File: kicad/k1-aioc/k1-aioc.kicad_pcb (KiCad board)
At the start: 2 copper layers, 21 x 31.5 mm, 47 parts, among them J1 12401832E402A, J2 Conn_01x07_Male, Q1 BC847BS, U1 MIC5330-SSYML, U2 STM32F373CBTx, Y1 8MHz/20pF

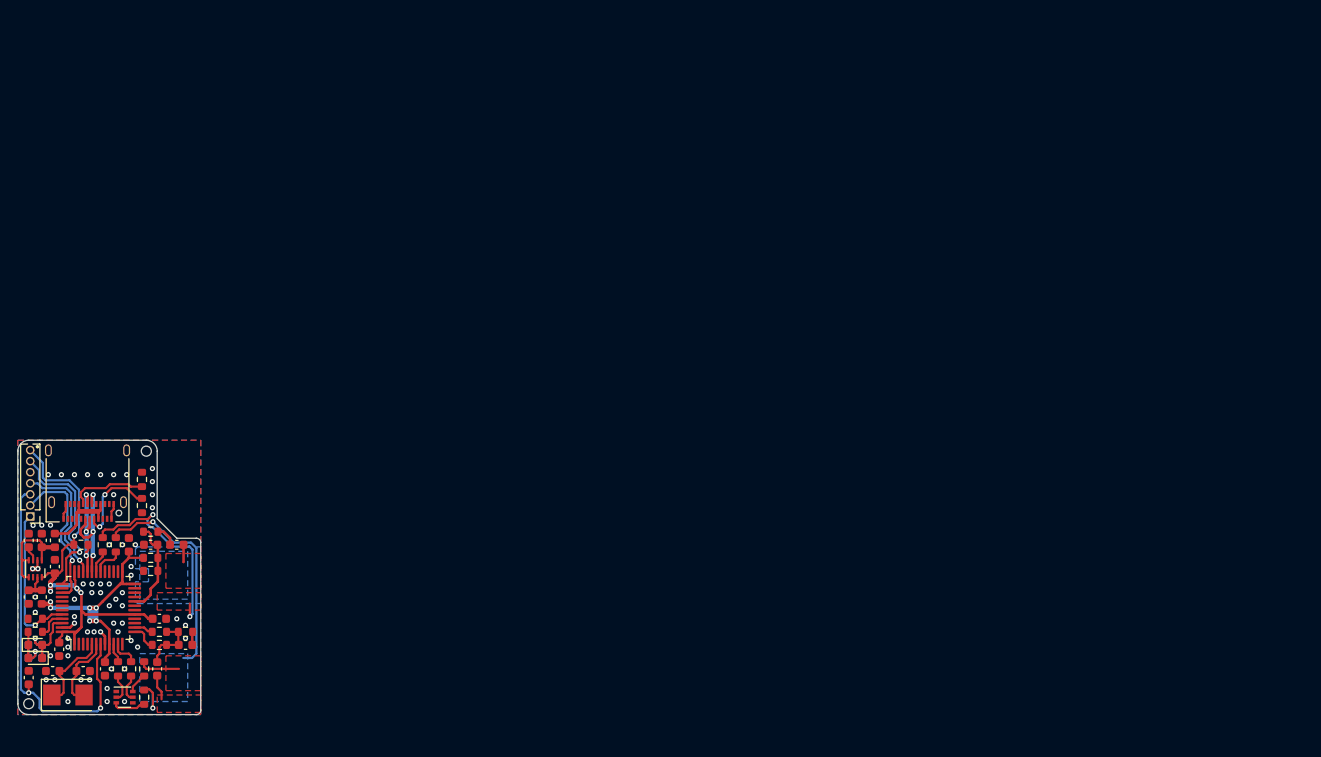
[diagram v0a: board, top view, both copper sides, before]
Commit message: Extensive PCB rework for new form factor
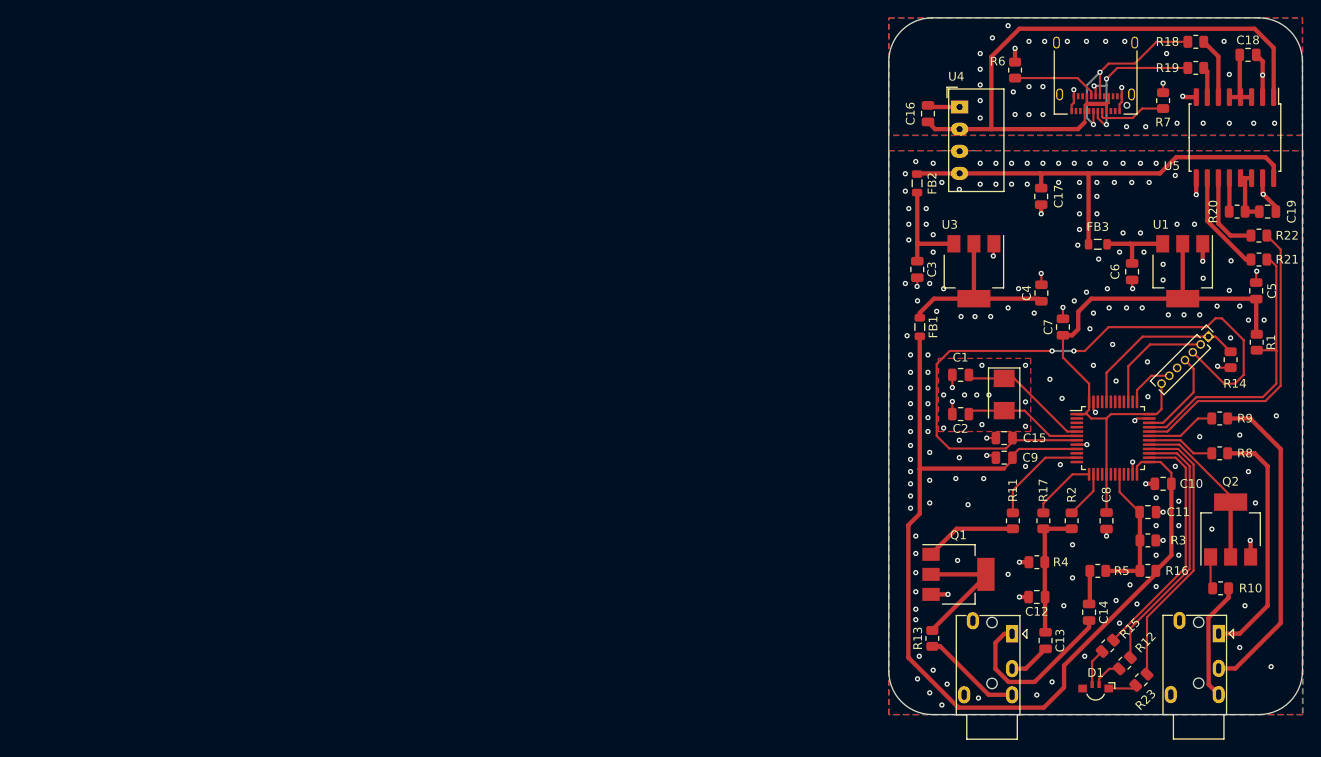
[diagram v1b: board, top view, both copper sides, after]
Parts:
- removed D2: RED, LED_SMD:LED_0603_1608Metric
- removed D3, D4: N.M., LED_SMD:LED_0603_1608Metric
- removed H1, H2: ToolingHole, AIOC:TOOLING-HOLE
- removed REF**: OSHW-Logo2_9.8x8mm_SilkScreen, Symbol:OSHW-Logo2_9.8x8mm_SilkScreen
- added C16: 4.7u/10V/X5R, Capacitor_SMD:C_0805_2012Metric, F.Cu at (208.0, 42.5)
- added C17: 4.7u/10V/X5R, Capacitor_SMD:C_0805_2012Metric, F.Cu at (221.0, 52.0)
- added C18: 100n, Capacitor_SMD:C_0805_2012Metric, F.Cu at (244.8, 35.8)
- added C19: 100n, Capacitor_SMD:C_0805_2012Metric, F.Cu at (247.0, 53.8)
- added FB2: 600R@100MHz, Inductor_SMD:L_0805_2012Metric, F.Cu at (206.8, 50.5)
- added J3: AUDIO, Connector_Audio:Jack_3.5mm_PJ320E_Horizontal, F.Cu at (217.7, 102.2)
- added J4: CAT, Connector_Audio:Jack_3.5mm_PJ320E_Horizontal, F.Cu at (241.4, 102.2)
- added Q2: PZT2222A, Package_TO_SOT_SMD:SOT-223-3_TabPin2, F.Cu at (242.8, 90.2)
- added R18: 24, Resistor_SMD:R_0805_2012Metric, F.Cu at (238.8, 34.2)
- added R19: 24, Resistor_SMD:R_0805_2012Metric, F.Cu at (238.8, 37.2)
- added R20: 5.1K, Resistor_SMD:R_0805_2012Metric, F.Cu at (243.5, 53.8)
- added R21: 24, Resistor_SMD:R_0805_2012Metric, F.Cu at (246.0, 59.2)
- added R22: 24, Resistor_SMD:R_0805_2012Metric, F.Cu at (246.0, 56.5)
- added R23: 220R, Resistor_SMD:R_0805_2012Metric, F.Cu at (232.5, 107.5)
- added U3: TLV1117LV-33, Package_TO_SOT_SMD:SOT-223-3_TabPin2, F.Cu at (213.3, 60.6)
- added U4: CRE1S0505SC, Converter_DCDC:Converter_DCDC_Murata_CRE1xxxxxxSC_THT, F.Cu at (211.6, 41.7)
- added U5: ADUM3160, Package_SO:SOIC-16W_7.5x10.3mm_P1.27mm, F.Cu at (243.2, 45.2)
- C1, C10, C11, C12, C13, C14, C15, C2, C4, C5, C6, C8, C9: footprint Capacitor_SMD:C_0603_1608Metric -> Capacitor_SMD:C_0805_2012Metric
- C3: value 100n -> 4.7u/10V/X5R; footprint Capacitor_SMD:C_0603_1608Metric -> Capacitor_SMD:C_0805_2012Metric
- C7: value 4.7u/10V/X5R -> 100n; footprint Capacitor_SMD:C_0603_1608Metric -> Capacitor_SMD:C_0805_2012Metric
- D1: value GREEN -> LED_RGBK; footprint LED_SMD:LED_0603_1608Metric -> LED_SMD:LED_Kingbright_APFA3010_3x1.5mm_Horizontal
- FB1: footprint Inductor_SMD:L_0603_1608Metric -> Inductor_SMD:L_0805_2012Metric
- FB3: renamed from FB2; footprint Inductor_SMD:L_0603_1608Metric -> Inductor_SMD:L_0805_2012Metric
- Q1: value BC847BS -> PZT2222A; footprint Package_TO_SOT_SMD:SOT-363_SC-70-6 -> Package_TO_SOT_SMD:SOT-223-3_TabPin2
- R1, R11, R14, R15, R16, R17, R2, R3, R4, R5, R6, R7, R8, R9: footprint Resistor_SMD:R_0603_1608Metric -> Resistor_SMD:R_0805_2012Metric
- R10: value 2.2K -> 24R; footprint Resistor_SMD:R_0603_1608Metric -> Resistor_SMD:R_0805_2012Metric
- R12: value 22R -> 220R; footprint Resistor_SMD:R_0603_1608Metric -> Resistor_SMD:R_0805_2012Metric
- R13: value 22R -> 24R; footprint Resistor_SMD:R_0603_1608Metric -> Resistor_SMD:R_0805_2012Metric
- U1: value MIC5330-SSYML -> TLV1117LV-33; footprint AIOC:Micrel_MLF-8-1EP_2x2mm_P0.5mm_EP0.6x1.2mm -> Package_TO_SOT_SMD:SOT-223-3_TabPin2
- moved C5 145.3 mm to (245.7, 62.8), turned to 90 degrees
- moved R14 140.4 mm to (242.8, 70.8), turned to 90 degrees
- moved R1 137.0 mm to (245.8, 68.8), turned to -90 degrees
- moved J2 136.8 mm to (240.2, 68.1), turned to -45 degrees
- moved U1 136.1 mm to (237.2, 60.6)
- moved R9 129.1 mm to (241.5, 77.5), turned to 180 degrees
- moved C6 128.9 mm to (231.4, 60.6), turned to -90 degrees
- moved R8 127.2 mm to (241.5, 81.5), turned to 180 degrees
- moved R10 126.9 mm to (241.6, 97.0), turned to 180 degrees
- moved R7 126.1 mm to (235.0, 41.0), turned to -90 degrees
- moved J1 124.9 mm to (227.2, 38.2)
- moved FB3 124.5 mm to (227.5, 57.5), turned to 180 degrees
- moved R15 123.2 mm to (228.6, 103.6), turned to 45 degrees
- moved D1 121.9 mm to (227.2, 108.5), turned to 180 degrees
- moved C8 121.2 mm to (228.5, 89.2)
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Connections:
- C4 pad 1: +3V3 -> Net-(C4-Pad1)
- C5 pad 1: Net-(C5-Pad1) -> +3V3
- C6 pad 1: /VIN -> Net-(C6-Pad1)
- D1 pad 2: Net-(D1-Pad2) -> GND
- FB1 pad 1: +3.3VA -> Net-(C4-Pad1)
- FB1 pad 2: Net-(C5-Pad1) -> +3.3VA
- FB3 pad 1: /VIN -> Net-(C6-Pad1)
- FB3 pad 2: /VBUS -> Net-(C17-Pad1)
- J1 pad A1: GND -> GNDREF
- J1 pad A12: GND -> GNDREF
- J1 pad A4: /VBUS -> Net-(U5-Pad1)
- J1 pad A6: /USB-DP -> Net-(J1-PadA6)
- J1 pad A7: /USB-DN -> Net-(J1-PadA7)
- J1 pad A9: /VBUS -> Net-(U5-Pad1)
- J1 pad B1: GND -> GNDREF
- J1 pad B12: GND -> GNDREF
- J1 pad B4: /VBUS -> Net-(U5-Pad1)
- J1 pad B6: /USB-DP -> Net-(J1-PadA6)
- J1 pad B7: /USB-DN -> Net-(J1-PadA7)
- J1 pad B9: /VBUS -> Net-(U5-Pad1)
- J1 pad S1: GND -> GNDREF
- Q1 pad 1: GND -> Net-(R11-Pad2)
- Q1 pad 2: Net-(Q1-Pad2) -> Net-(R13-Pad2)
- Q1 pad 3: Net-(Q1-Pad3) -> GND
- R1 pad 2: /USB-DP -> /USB-DP-D
- R10 pad 1: /PTT2 -> /COS
- R10 pad 2: Net-(Q1-Pad2) -> Net-(Q2-Pad1)
- R11 pad 2: Net-(Q1-Pad5) -> Net-(R11-Pad2)
- R12 pad 1: /RADIO-VP-PTT2 -> Net-(D1-Pad4)
- R12 pad 2: Net-(Q1-Pad6) -> /LED_B
- R13 pad 1: /RADIO-RX-PTT1 -> /RADIO-PTT
- R13 pad 2: Net-(Q1-Pad3) -> Net-(R13-Pad2)
- R15 pad 1: Net-(D1-Pad1) -> Net-(D1-Pad3)
- R15 pad 2: Net-(R15-Pad2) -> /LED_G
- R6 pad 1: GND -> GNDREF
- R7 pad 1: GND -> GNDREF
- R8 pad 1: /RADIO-RX-PTT1 -> /RADIO-RX
- U1 pad 1: /VIN -> GND
- U1 pad 2: GND -> +3V3
- U1 pad 3: Net-(C3-Pad1) -> Net-(C6-Pad1)
- U2 pad 10: /PTT2 -> unconnected-(U2-Pad10)
- U2 pad 26: unconnected-(U2-Pad26) -> /LED_G
- U2 pad 27: unconnected-(U2-Pad27) -> /LED_B
- U2 pad 28: unconnected-(U2-Pad28) -> /LED_R
- U2 pad 29: unconnected-(U2-Pad29) -> Net-(U2-Pad29)
- U2 pad 32: /USB-DN -> /USB-DN-D
- U2 pad 33: /USB-DP -> /USB-DP-D
- U2 pad 45: Net-(R15-Pad2) -> unconnected-(U2-Pad45)
- U2 pad 46: Net-(D1-Pad2) -> unconnected-(U2-Pad46)
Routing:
- net +3.3VA: track 30.8 -> 113.3 mm, vias 6 -> 0
- net Net-(U5-Pad1): track 0.00 -> 77.2 mm
- net Net-(C17-Pad1): track 0.00 -> 53.4 mm
- net /USB-DN-D: track 0.00 -> 35.2 mm
- net /USB-DP-D: track 0.00 -> 34.3 mm
- net /NRST: track 43.4 -> 75.9 mm
- net /LED_R: track 0.00 -> 32.1 mm
- net /LED_B: track 0.00 -> 30.1 mm
- net /RADIO-RX-PTT1: track 30.0 -> 0.00 mm, vias 2 -> 0
- net GND: track 9.36 -> 38.8 mm, vias 62 -> 196
- net /RADIO-RX: track 0.00 -> 28.2 mm
- net /LED_G: track 0.00 -> 27.9 mm
- net Net-(J1-PadA7): track 0.00 -> 22.8 mm, vias 0 -> 2
- net Net-(C4-Pad1): track 0.00 -> 21.2 mm
- net +3V3: track 51.0 -> 71.0 mm, vias 5 -> 0
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- added copper zone on B.Cu, net GNDREF
- added copper zone on F.Cu, net GNDREF
- removed copper zone on F.Cu, net /RADIO-MIC
- removed copper zone on B.Cu, net /RADIO-RX-PTT1
- removed copper zone on F.Cu, net /RADIO-SPK
- removed copper zone on F.Cu, net /RADIO-TX
- removed copper zone on F.Cu, net /RADIO-VP-PTT2
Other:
- board size 21 x 31.5 mm -> 47.5 x 80 mm
- board text removed: "2.5mm"
- board text removed: "3.5mm"
- board text removed: "3V3"
- board text removed: "AIOC V1.0"
- board text removed: "BLD"
- board text removed: "BOOT"
- board text removed: "GND"
- board text removed: "K1-Conn."
- board text removed: "RST"
- board text removed: "S. Kueppers"
- board text removed: "SWC"
- board text removed: "SWD"
- board text removed: "SWO"
